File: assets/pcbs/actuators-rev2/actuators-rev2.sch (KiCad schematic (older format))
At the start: 14 parts, among them J2 Screw_Terminal_01x02, J3 Screw_Terminal_01x02, J5 40HAT, J6 Conn_01x02, J7 Screw_Terminal_01x02, U1 ULN2003A, U2 PDQ15-Q24-S5-D

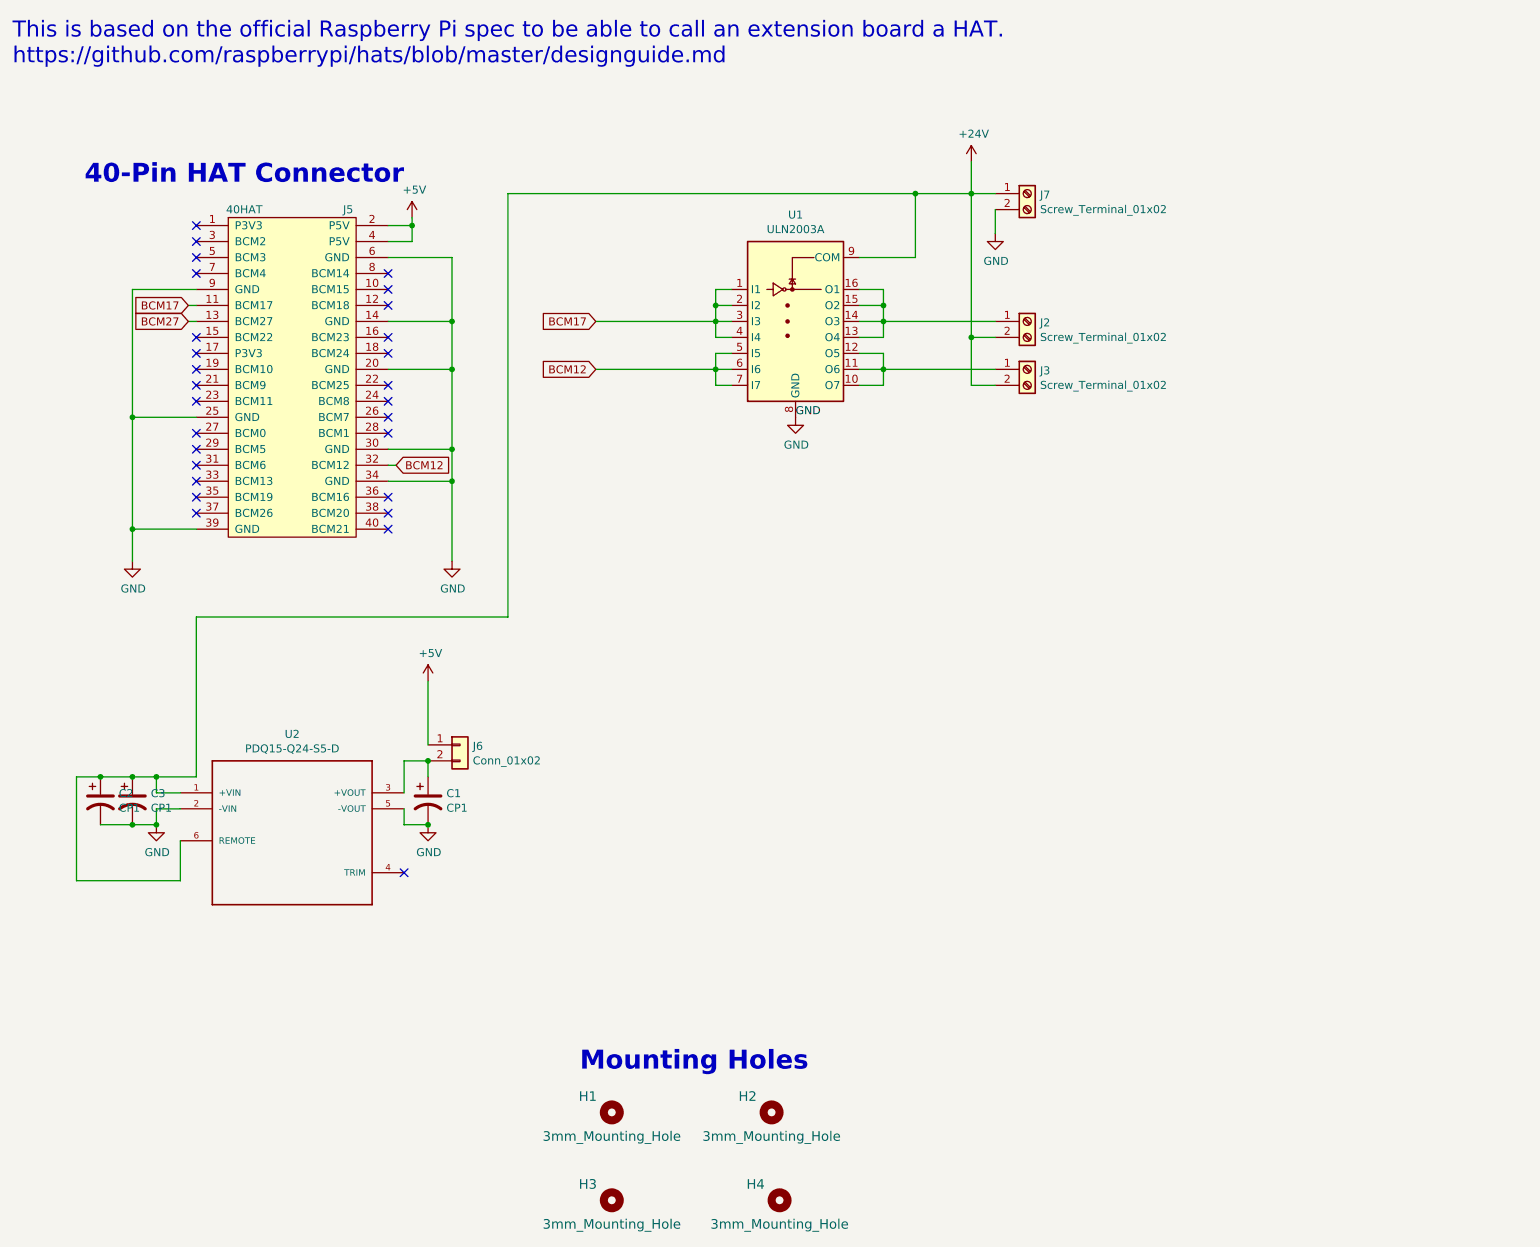
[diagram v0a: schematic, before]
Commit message: revised, added schematic images
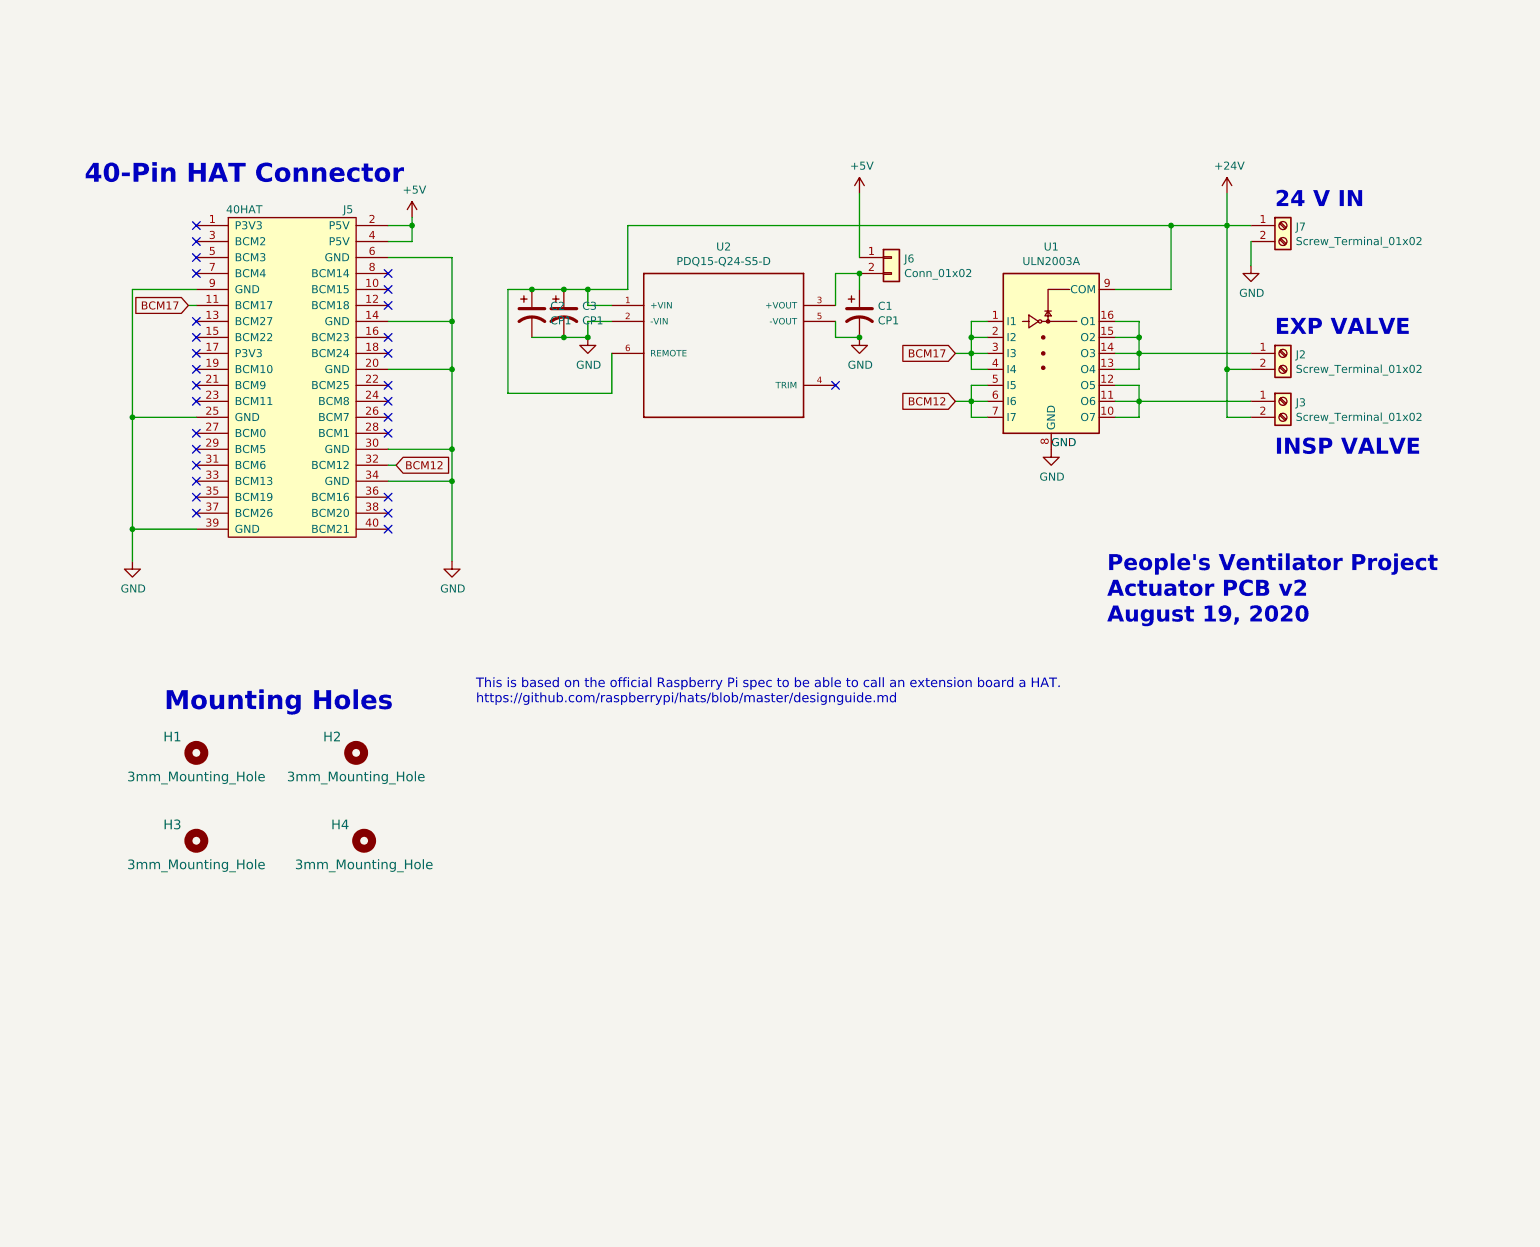
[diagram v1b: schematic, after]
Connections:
- net BCM27: no longer names the net of J5.13 (BCM27)
- no-connect marks 28 -> 29
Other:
- note added: "24 V IN"
- note added: "EXP VALVE"
- note added: "INSP VALVE"
- note added: "People's Ventilator Project\nActuator PCB v2\nAugust 19, 2020"
- moved on the sheet: C1, C2, C3, H1, H2, H3, H4, J2, J3, J6, J7, U1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
